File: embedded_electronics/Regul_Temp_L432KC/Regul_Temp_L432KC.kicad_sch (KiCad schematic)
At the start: 28 parts, among them J1 TRIM_CONSIGNE, J10 MOT_OUT, J11 Digilent Motor, J12 2.54 motor, J2 Temp_In, J3 POWER_IN_5V, J4 SW_MODE, J5 OUT_to_BNC, J6 Consigne, J7 Erreur, J8 OLED, J9 POWER_MOTOR_6V, Q1 IRL540N, U1 LM358, U2 NUCLEO-L432KC

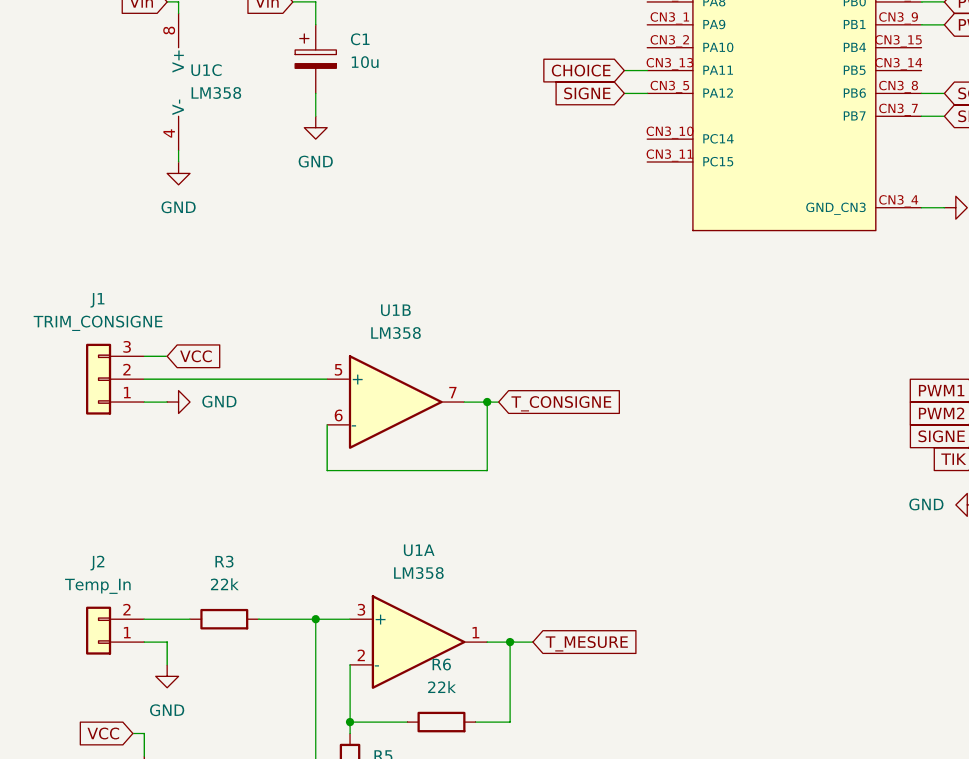
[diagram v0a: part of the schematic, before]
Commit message: Update Regul temp
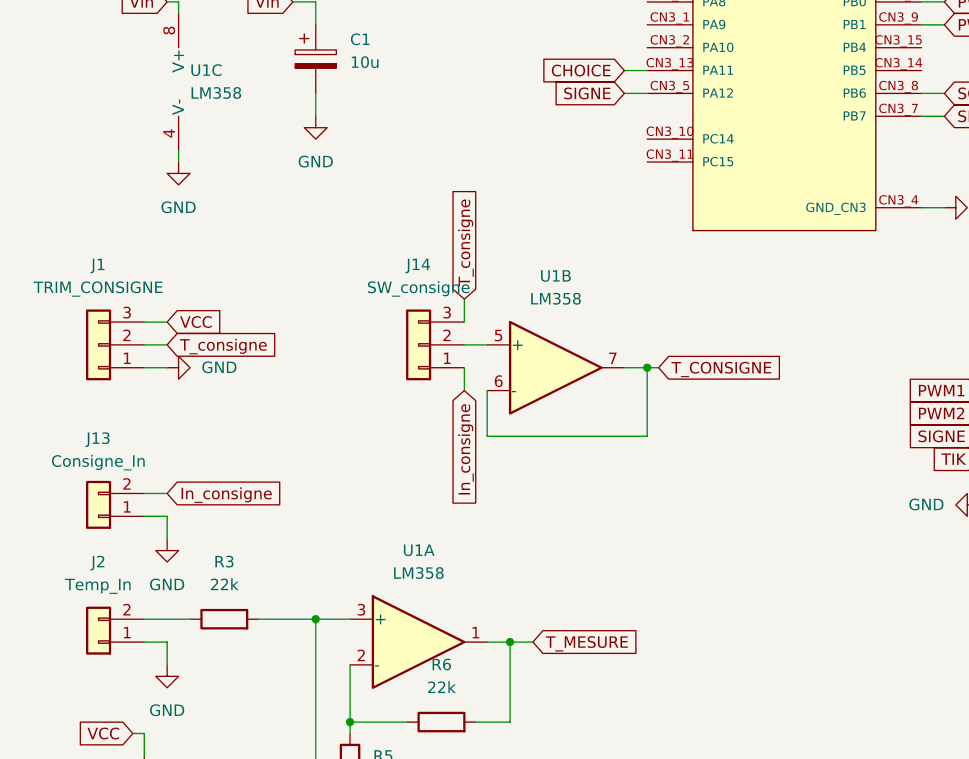
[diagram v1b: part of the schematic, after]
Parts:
- added J13: Consigne_In, Connector_PinSocket_2.54mm:PinSocket_1x02_P2.54mm_Vertical, symbol Connector_Generic:Conn_01x02
- added J14: SW_consigne, Connector_PinSocket_2.54mm:PinSocket_1x03_P2.54mm_Vertical, symbol Connector_Generic:Conn_01x03
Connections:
- net GND: now also J13.1 (Pin_1)
- net at U1.5 (+): now also J14.2 (Pin_2); no longer J1.2 (Pin_2)
- new net In_consigne: J13.2 (Pin_2), J14.1 (Pin_1)
- new net T_consigne: J1.2 (Pin_2), J14.3 (Pin_3)
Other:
- moved on the sheet: J1, U1B
